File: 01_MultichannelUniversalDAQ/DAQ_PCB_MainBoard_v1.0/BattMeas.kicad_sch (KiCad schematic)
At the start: 12 parts, among them U2 AMC1200BDWV, U7 NCP163ASN350T1G

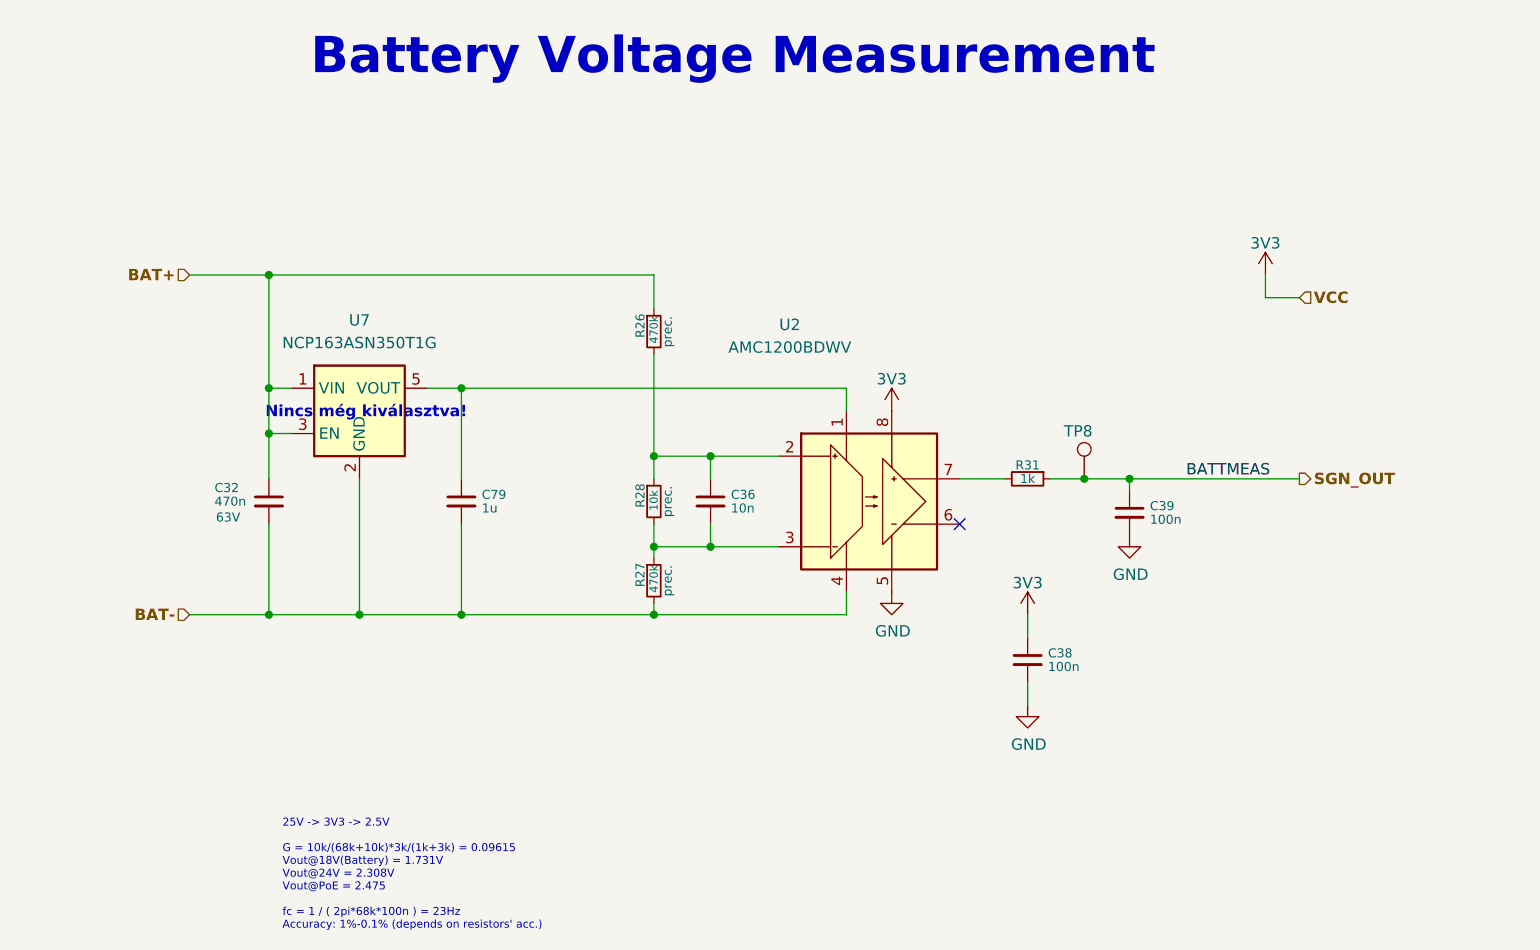
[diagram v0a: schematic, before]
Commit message: new power concept
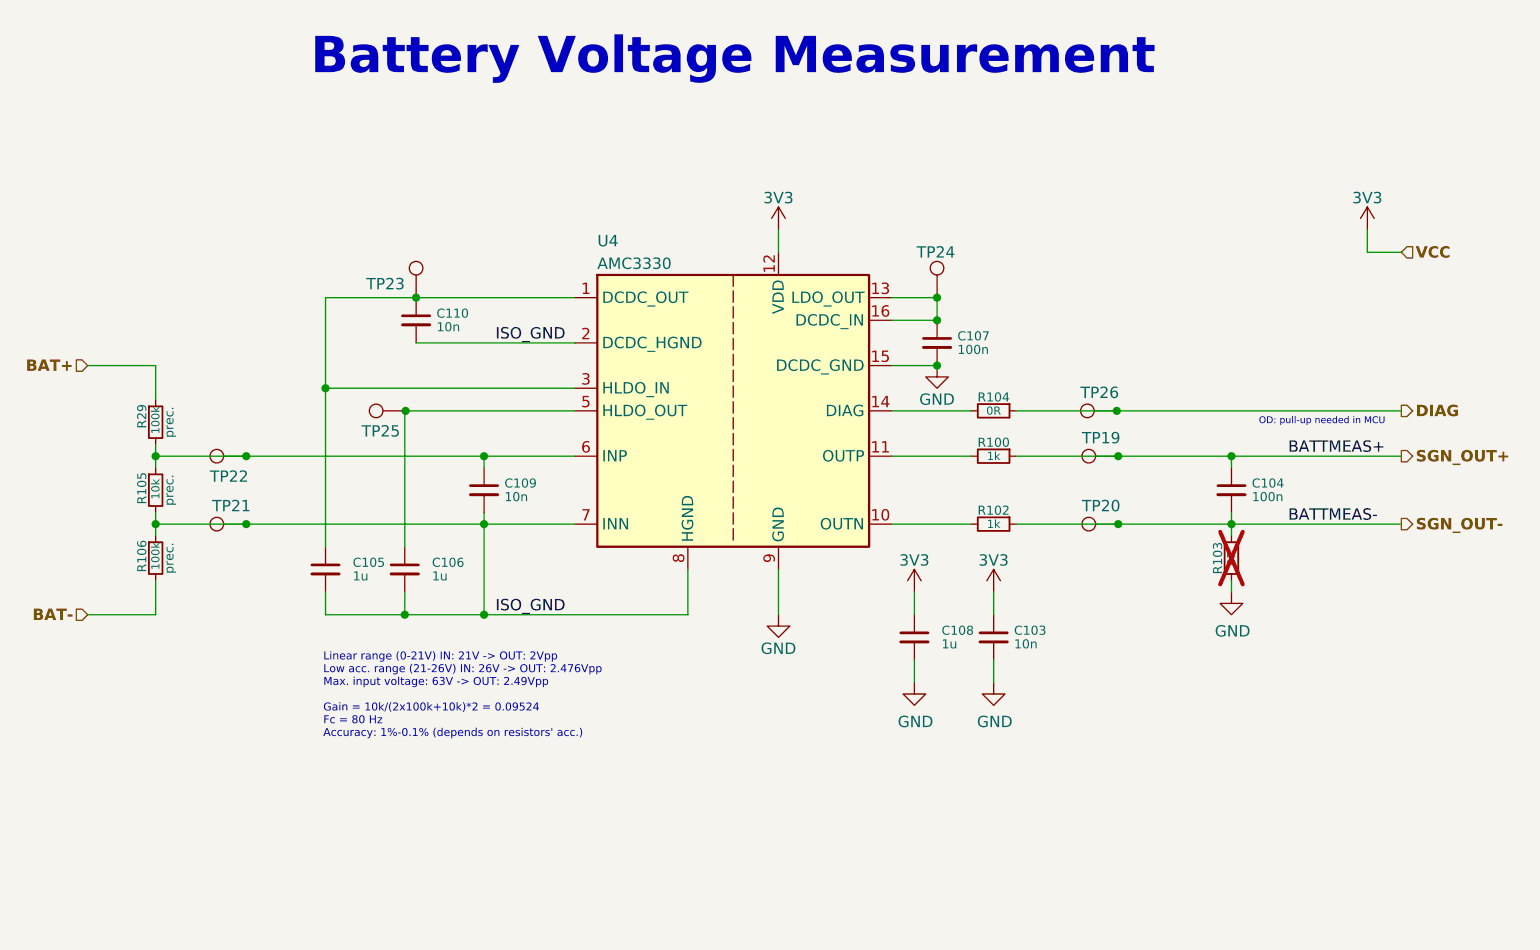
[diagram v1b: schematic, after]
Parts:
- removed C32: 470n, Capacitor_SMD:C_1206_3216Metric_Pad1.33x1.80mm_HandSolder, symbol Device:C_Small
- removed C36: 10n, Capacitor_SMD:C_0603_1608Metric_Pad1.08x0.95mm_HandSolder, symbol Device:C_Small
- removed C38, C39: 100n, Capacitor_SMD:C_0603_1608Metric_Pad1.08x0.95mm_HandSolder, symbol Device:C_Small
- removed C79: 1u, Capacitor_SMD:C_0603_1608Metric_Pad1.08x0.95mm_HandSolder, symbol Device:C_Small
- removed R26, R27: 470k, Resistor_SMD:R_0603_1608Metric_Pad0.98x0.95mm_HandSolder, symbol Device:R_Small
- removed R28: 10k, Resistor_SMD:R_0603_1608Metric_Pad0.98x0.95mm_HandSolder, symbol Device:R_Small
- removed R31: 1k, Resistor_SMD:R_0603_1608Metric_Pad0.98x0.95mm_HandSolder, symbol Device:R_Small
- removed TP8: TestPoint, TestPoint:TestPoint_Pad_D1.0mm, symbol Connector:TestPoint
- removed U2: AMC1200BDWV, Package_SO:SOIC-8_7.5x5.85mm_P1.27mm, symbol Isolator_Analog:AMC1200BDWV
- removed U7: NCP163ASN350T1G, Package_TO_SOT_SMD:SOT-23-5, symbol Regulator_Linear:NCP163ASN350T1G
- added C103, C109, C110: 10n, Capacitor_SMD:C_0603_1608Metric_Pad1.08x0.95mm_HandSolder, symbol Device:C_Small
- added C104, C107: 100n, Capacitor_SMD:C_0603_1608Metric_Pad1.08x0.95mm_HandSolder, symbol Device:C_Small
- added C105, C106, C108: 1u, Capacitor_SMD:C_0603_1608Metric_Pad1.08x0.95mm_HandSolder, symbol Device:C_Small
- added R100, R102: 1k, Resistor_SMD:R_0603_1608Metric_Pad0.98x0.95mm_HandSolder, symbol Device:R_Small
- added R103, R104: 0R, Resistor_SMD:R_0603_1608Metric_Pad0.98x0.95mm_HandSolder, symbol Device:R_Small
- added R105: 10k, Resistor_SMD:R_0603_1608Metric_Pad0.98x0.95mm_HandSolder, symbol Device:R_Small
- added R106, R29: 100k, Resistor_SMD:R_0805_2012Metric_Pad1.20x1.40mm_HandSolder, symbol Device:R_Small
- added TP19, TP20, TP21, TP22, TP23, TP24, TP25, TP26: TestPoint, TestPoint:TestPoint_Pad_D1.0mm, symbol Connector:TestPoint
- added U4: AMC3330, Package_SO:SOIC-16W_7.5x10.3mm_P1.27mm, symbol Isolator_Analog:AMC3330
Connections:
- net 3V3: now also C103.1, C108.1, U4.12 (VDD)
- net BAT+: now also R29.1
- net BAT-: now also R106.2
- net GND: now also C103.2, C107.2, C108.2, R103.2, U4.15 (DCDC_GND), U4.9 (GND)
- new net: C105.1, C110.1, TP23.1, U4.1 (DCDC_OUT), U4.3 (HLDO_IN)
- new net: R100.2, U4.11 (OUTP)
- new net: C109.1, R105.1, R29.2, TP22.1, U4.6 (INP)
- new net: R104.2, U4.14 (DIAG)
- new net: R102.2, U4.10 (OUTN)
- new net: C106.1, TP25.1, U4.5 (HLDO_OUT)
- new net: C107.1, TP24.1, U4.13 (LDO_OUT), U4.16 (DCDC_IN)
- new net DIAG: R104.1, TP26.1
- new net ISO_GND: C105.2, C106.2, C109.2, C110.2, R105.2, R106.1, TP21.1, U4.2 (DCDC_HGND), U4.7 (INN), U4.8 (HGND)
- new net SGN_OUT+: C104.1, R100.1, TP19.1
- new net SGN_OUT-: C104.2, R102.1, R103.1, TP20.1
- no-connect marks 1 -> 0
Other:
- note added: "Linear range (0-21V) IN: 21V -> OUT: 2Vpp Low acc. range (21-26V) IN: 26V -> OUT: 2.476Vpp Max. input voltage: 63V -> OUT: 2.49Vpp Gain = 10k/(2x100k+10k)*2 = 0.09524 Fc = 80 Hz Accuracy: 1%-0.1% (depends on resistors' acc.)"
- note added: "OD: pull-up needed in MCU"
- note removed: "25V -> 3V3 -> 2.5V G = 10k/(68k+10k)*3k/(1k+3k) = 0.09615 Vout@18V(Battery) = 1.731V Vout@24V = 2.308V Vout@PoE = 2.475 fc = 1 / ( 2pi*68k*100n ) = 23Hz Accuracy: 1%-0.1% (depends on resistors' acc.)"
- note removed: "Nincs még kiválasztva!"
